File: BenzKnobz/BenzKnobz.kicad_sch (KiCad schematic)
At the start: 115 parts, among them J1 Barrel_Jack, J10 I2C_STANDARDJS-1MM, J2 MIDI OUT, J3 MIDI IN, J4 MJ-3502, J5 MJ-3502, J6 MJ-3502, J7 MJ-3502, J8 MJ-3502, J9 MJ-3502, SW1 SW_MEC_5E, SW2 SW_MEC_5E, SW3 SW_MEC_5E, SW4 SW_MEC_5E, SW5 SW_MEC_5E, SW6 SW_MEC_5E, U1 teensy 4.0, U10 6N138, U2 TXB0108DQSR, U3 74HC4051, U4 74HC4051, U5 74HC4051, U6 74HC4051, U7 74HC4051, U8 74HC4051, U9 74HC4051

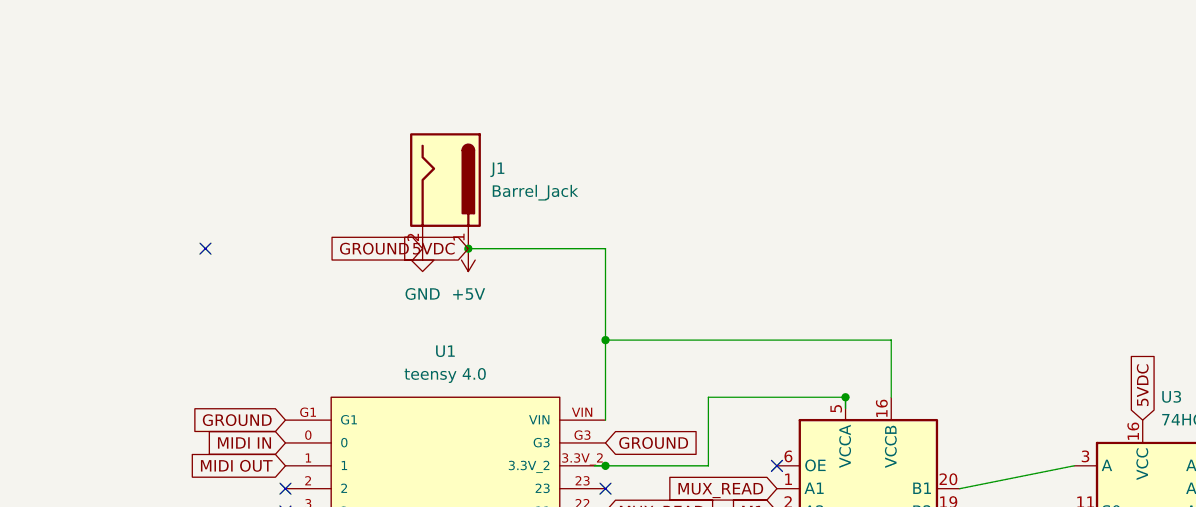
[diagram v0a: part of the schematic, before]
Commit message: circuit/board
finalizing power regulation
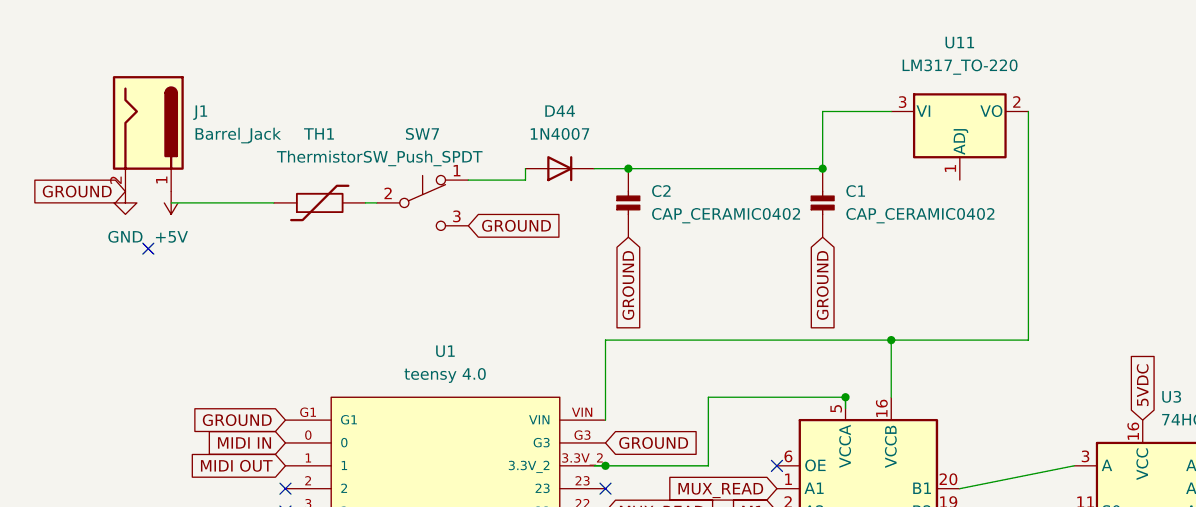
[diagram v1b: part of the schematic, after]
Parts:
- added C1, C2: CAP_CERAMIC0402, Capacitor_THT:C_Disc_D4.3mm_W1.9mm_P5.00mm, symbol BenzKnobz-eagle-import:CAP_CERAMIC0402
- added D44: 1N4007, Diode_THT:D_DO-41_SOD81_P10.16mm_Horizontal, symbol Diode:1N4007
- added SW7: SW_Push_SPDT, Button_Switch_THT:SW_PUSH_6mm, symbol Switch:SW_Push_SPDT
- added TH1: Thermistor, Capacitor_THT:C_Disc_D9.0mm_W5.0mm_P7.50mm, symbol Device:Thermistor
- added U11: LM317_TO-220, Package_TO_SOT_THT:TO-220-3_Vertical, symbol Regulator_Linear:LM317_TO-220
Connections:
- net +5V: no longer D1.3 (VDD), D10.3 (VDD), D11.3 (VDD), D12.3 (VDD), D13.3 (VDD), D14.3 (VDD), D15.3 (VDD), D16.3 (VDD), D17.3 (VDD), D18.3 (VDD), D19.3 (VDD), D2.3 (VDD), D20.3 (VDD), D21.3 (VDD), D22.3 (VDD), D23.3 (VDD), D24.3 (VDD), D25.3 (VDD), D26.3 (VDD), D27.3 (VDD), D28.3 (VDD), D29.3 (VDD), D3.3 (VDD), D30.3 (VDD), D31.3 (VDD), D32.3 (VDD), D33.3 (VDD), D34.3 (VDD), D35.3 (VDD), D36.3 (VDD), D37.3 (VDD), D38.3 (VDD), D39.3 (VDD), D4.3 (VDD), D40.3 (VDD), D41.3 (VDD), D42.3 (VDD), D5.3 (VDD), D6.3 (VDD), D7.3 (VDD), D8.3 (VDD), D9.3 (VDD), J10.2 (VCC), R10.1, R11.1, R12.1, R13.1, R14.1, R15.1, R16.1, R17.1, R18.1, R19.1, R2.1, R20.1, R21.1, R22.1, R23.1, R24.1, R25.1, R26.1, R27.1, R28.1, R29.1, R30.1, R31.1, R32.1, R33.1, R34.1, R35.1, R36.1, R37.1, R38.1, R39.1, R4.1, R40.1, R41.1, R42.1, R43.1, R44.1, R45.1, R46.1, R5.1, R6.1, R7.1, R8.1, R9.1, SW1.1, SW2.1, SW3.1, SW4.1, SW5.1, SW6.1, U1.VIN, U10.8 (VCC), U2.16 (VCCB), U3.16 (VCC), U4.16 (VCC), U5.16 (VCC), U6.16 (VCC), U7.16 (VCC), U8.16 (VCC), U9.16 (VCC)
- net GND: now also C1.2 (P$2), C2.2 (P$2), SW7.3 (C)
- new net: U1.VIN, U11.2 (VO), U2.16 (VCCB)
- new net: C1.1 (P$1), C2.1 (P$1), D44.1 (K), U11.3 (VI)
- new net: D44.2 (A), SW7.1 (A)
- new net: SW7.2 (B), TH1.2
- new net 5VDC: D1.3 (VDD), D10.3 (VDD), D11.3 (VDD), D12.3 (VDD), D13.3 (VDD), D14.3 (VDD), D15.3 (VDD), D16.3 (VDD), D17.3 (VDD), D18.3 (VDD), D19.3 (VDD), D2.3 (VDD), D20.3 (VDD), D21.3 (VDD), D22.3 (VDD), D23.3 (VDD), D24.3 (VDD), D25.3 (VDD), D26.3 (VDD), D27.3 (VDD), D28.3 (VDD), D29.3 (VDD), D3.3 (VDD), D30.3 (VDD), D31.3 (VDD), D32.3 (VDD), D33.3 (VDD), D34.3 (VDD), D35.3 (VDD), D36.3 (VDD), D37.3 (VDD), D38.3 (VDD), D39.3 (VDD), D4.3 (VDD), D40.3 (VDD), D41.3 (VDD), D42.3 (VDD), D5.3 (VDD), D6.3 (VDD), D7.3 (VDD), D8.3 (VDD), D9.3 (VDD), J10.2 (VCC), R10.1, R11.1, R12.1, R13.1, R14.1, R15.1, R16.1, R17.1, R18.1, R19.1, R2.1, R20.1, R21.1, R22.1, R23.1, R24.1, R25.1, R26.1, R27.1, R28.1, R29.1, R30.1, R31.1, R32.1, R33.1, R34.1, R35.1, R36.1, R37.1, R38.1, R39.1, R4.1, R40.1, R41.1, R42.1, R43.1, R44.1, R45.1, R46.1, R5.1, R6.1, R7.1, R8.1, R9.1, SW1.1, SW2.1, SW3.1, SW4.1, SW5.1, SW6.1, U10.8 (VCC), U3.16 (VCC), U4.16 (VCC), U5.16 (VCC), U6.16 (VCC), U7.16 (VCC), U8.16 (VCC), U9.16 (VCC)
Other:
- moved on the sheet: J1

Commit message: kicad again
might need to restart layout
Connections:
- net 5VDC: now also SW1.2, SW2.2, SW3.2, SW4.2, SW5.2, SW6.2, TH1.1
- net B1_8: now also SW1.3 (K)
- net B2_8: now also SW2.3 (K)
- net B3_8: now also SW3.3 (K)
- net B4_8: now also SW4.3 (K)
- net B5_8: now also SW5.3 (K)
- net B6_8: now also SW6.3 (K)
- net MuxBD1: now reaches U3.13 (A0), U4.3 (A)
- net MuxBD5: now reaches U3.1 (A4), U9.3 (A)
- net MuxA3: now reaches U2.17 (B4), U3.9 (S2)
- net MuxA2: now reaches U2.18 (B3), U3.10 (S1)
- net MuxA1: now reaches U2.19 (B2), U3.11 (S0)
- net MUX_OUT: now reaches U2.20 (B1), U3.3 (A)
- net MuxBD2: now reaches U3.14 (A1), U5.3 (A)
- net MuxBD3: now reaches U3.15 (A2), U6.3 (A)
- net MuxBD6: now reaches U3.5 (A5), U8.3 (A)
- net MuxBD4: now reaches U3.12 (A3), U7.3 (A)
- no-connect marks 38 -> 25
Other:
- moved on the sheet: J10, J4, J5, J6, J7, J8, J9, U3
